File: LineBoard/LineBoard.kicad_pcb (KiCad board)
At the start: 2 copper layers, 123.1 x 70 mm, 63 parts, among them IC1 S7136, IC2 S7136, J1 side_l, J2 side_l, J3 Conn_01x18_Pin, Q1 PT17-21B/L41/TR8, Q10 PT17-21B/L41/TR8, Q11 PT17-21B/L41/TR8, Q12 PT17-21B/L41/TR8, Q13 PT17-21B/L41/TR8, Q2 PT17-21B/L41/TR8, Q3 PT17-21B/L41/TR8, Q4 PT17-21B/L41/TR8, Q5 PT17-21B/L41/TR8, Q6 PT17-21B/L41/TR8, Q7 PT17-21B/L41/TR8, Q8 PT17-21B/L41/TR8, Q9 PT17-21B/L41/TR8

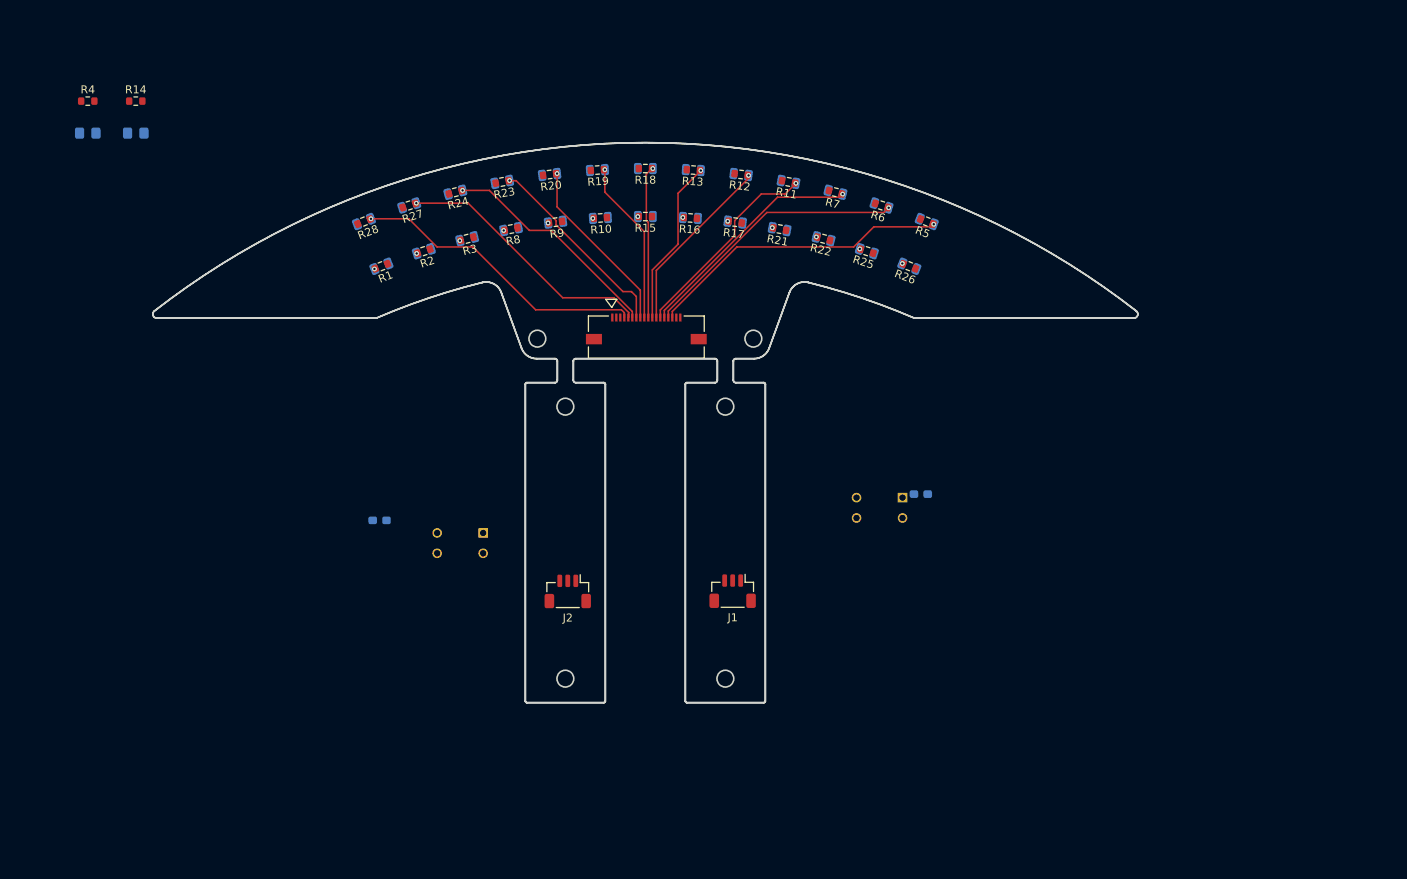
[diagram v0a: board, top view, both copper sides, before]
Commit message: 基板完成
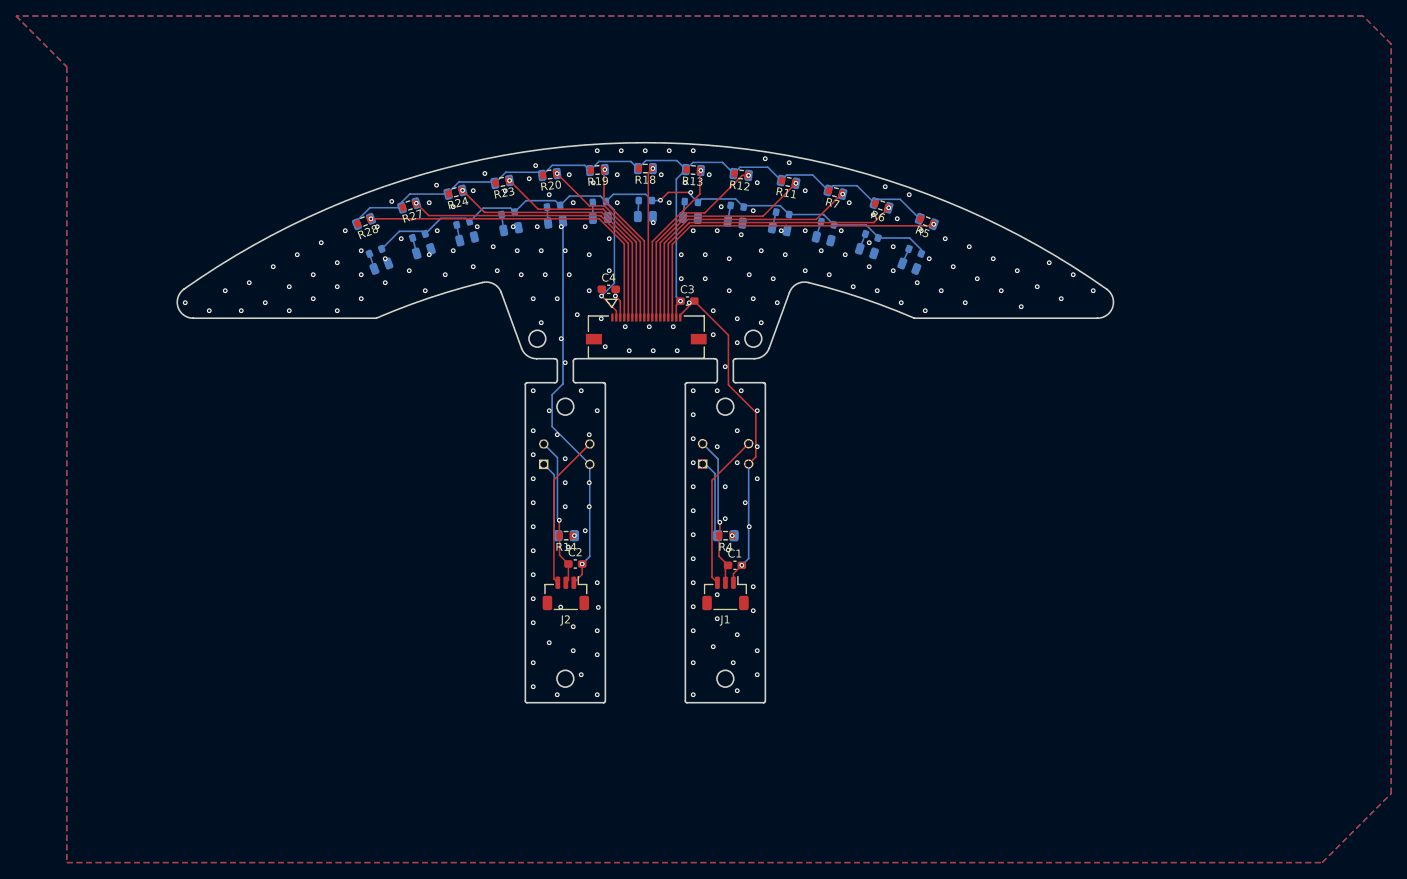
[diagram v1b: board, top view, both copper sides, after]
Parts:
- added C3: 0.1u, Capacitor_SMD:C_0603_1608Metric_Pad1.08x0.95mm_HandSolder, F.Cu at (133.0, 81.0)
- added C4: 0.1u, Capacitor_SMD:C_0603_1608Metric_Pad1.08x0.95mm_HandSolder, F.Cu at (123.1, 79.5)
- C1, C2: moved to F.Cu
- R1, R10, R15, R16, R17, R2, R21, R22, R25, R26, R3, R8, R9: moved to B.Cu
- moved R4 96.5 mm to (137.7, 110.3), turned to 180 degrees
- moved D14 94.3 mm to (137.8, 110.3)
- moved R14 76.5 mm to (117.8, 110.3), turned to 180 degrees
- moved D15 73.7 mm to (117.8, 110.3)
- moved C2 25.1 mm to (118.9, 113.9), turned to 0 degrees
- moved C1 24.9 mm to (138.9, 114.0), turned to 0 degrees
- moved IC1 20.4 mm to (137.7, 100.1), turned to 0 degrees
- moved IC2 17.4 mm to (117.9, 100.1), turned to 0 degrees
- moved R21 2.00 mm to (144.9, 70.0)
- moved R8 2.00 mm to (110.5, 70.0)
- moved R22 2.00 mm to (150.5, 71.3)
- moved R3 2.00 mm to (104.9, 71.3)
- moved R26 2.00 mm to (161.4, 74.8)
- moved R1 2.00 mm to (94.0, 74.8)
- moved R15 2.00 mm to (127.7, 68.4)
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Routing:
- net +5V: track 0.00 -> 132.1 mm, vias 0 -> 5
- net +3V3: track 0.00 -> 101.5 mm, vias 0 -> 1
- net GND: track 0.00 -> 94.7 mm, vias 0 -> 227
- net Net-(IC1-VOUT): track 0.00 -> 19.6 mm
- net Net-(IC2-VOUT): track 0.00 -> 19.4 mm
- net Net-(D14-K): track 0.00 -> 9.94 mm
- net Net-(D15-K): track 0.00 -> 9.65 mm
- net /VOUT13: track 37.1 -> 42.2 mm
- net /VOUT11: track 28.2 -> 33.3 mm
- net /VOUT12: track 32.9 -> 37.9 mm
- net /VOUT2: track 33.7 -> 38.6 mm
- net /VOUT1: track 37.9 -> 42.8 mm
- net /VOUT3: track 29.2 -> 34.0 mm
- net /VOUT4: track 25.5 -> 29.4 mm
- net /VOUT10: track 24.9 -> 28.5 mm
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- added copper zone on B.Cu, net GND
- added copper zone on F.Cu, net GND
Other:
- board size 123.1 x 70 mm -> 117 x 70 mm
